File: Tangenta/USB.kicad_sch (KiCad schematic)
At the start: 31 parts, among them J12 907-211A1019D10200, J13 906-861A2116D10210, U8 USB2514B-I_M2, X1 X322524MOB4SI

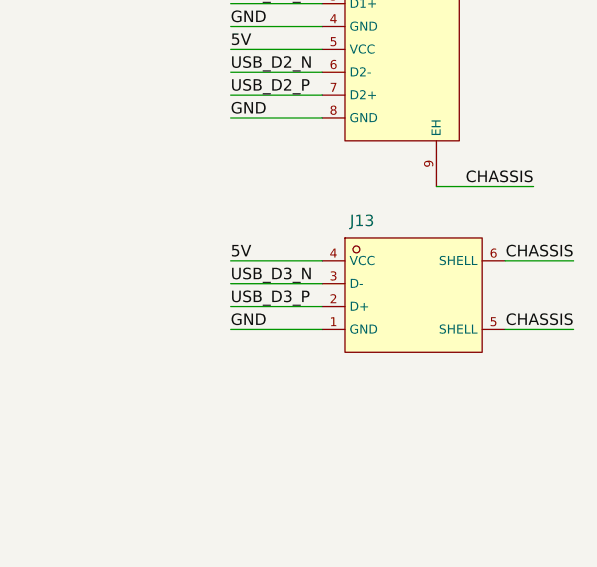
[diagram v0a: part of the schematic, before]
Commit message: ...
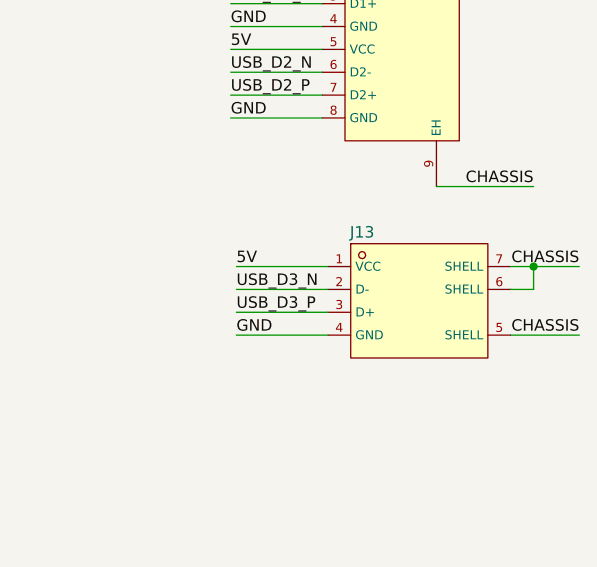
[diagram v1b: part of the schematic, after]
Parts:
- removed J13: 906-861A2116D10210, USB_VERTICAL:USB_Vertical, symbol USB_VERTICAL:906-861A2116D10210
- added J13: 906-151A1058D10200, USB_VERTICAL_BLUE:USB_VERTICAL_BLUE, symbol USB_VERTICAL_BLUE:906-151A1058D10200
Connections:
- net 5V: now also J13.1 (VCC)
- net CHASSIS: now also J13.5 (SHELL), J13.6 (SHELL), J13.7 (SHELL)
- net GNDREF: now also J13.4 (GND)
- net USB_D3_N: now also J13.2 (D-)
- net USB_D3_P: now also J13.3 (D+)
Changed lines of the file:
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@@
   (junction (at 114.3 177.8) (diameter 0) (color 0 0 0 0)
   )
+  (junction (at 279.4 88.9) (diameter 0) (color 0 0 0 0)
+  )
   (junction (at 95.25 168.91) (diameter 0) (color 0 0 0 0)
   )
@@
     (stroke (width 0) (type default))
   )
-  (wire (pts (xy 276.225 95.885) (xy 283.845 95.885))
+  (wire (pts (xy 276.86 96.52) (xy 284.48 96.52))
     (stroke (width 0) (type default))
   )
@@
     (stroke (width 0) (type default))
   )
-  (wire (pts (xy 276.225 88.265) (xy 283.845 88.265))
+  (wire (pts (xy 276.86 88.9) (xy 279.4 88.9))
     (stroke (width 0) (type default))
   )
@@
     (stroke (width 0) (type default))
   )
+  (wire (pts (xy 276.86 91.44) (xy 279.4 91.44))
+    (stroke (width 0) (type default))
+  )
   (wire (pts (xy 49.53 85.09) (xy 58.42 85.09))
     (stroke (width 0) (type default))
@@
     (stroke (width 0) (type default))
   )
-  (wire (pts (xy 245.745 95.885) (xy 255.905 95.885))
+  (wire (pts (xy 246.38 96.52) (xy 256.54 96.52))
     (stroke (width 0) (type default))
   )
@@
     (stroke (width 0) (type default))
   )
-  (wire (pts (xy 245.745 88.265) (xy 255.905 88.265))
+  (wire (pts (xy 246.38 88.9) (xy 256.54 88.9))
     (stroke (width 0) (type default))
   )
@@
     (stroke (width 0) (type default))
   )
-  (wire (pts (xy 245.745 90.805) (xy 255.905 90.805))
+  (wire (pts (xy 246.38 91.44) (xy 256.54 91.44))
     (stroke (width 0) (type default))
   )
@@
     (stroke (width 0) (type default))
   )
+  (wire (pts (xy 279.4 88.9) (xy 284.48 88.9))
+    (stroke (width 0) (type default))
+  )
   (wire (pts (xy 48.895 59.69) (xy 58.42 59.69))
     (stroke (width 0) (type default))
@@
     (stroke (width 0) (type default))
   )
-  (wire (pts (xy 245.745 93.345) (xy 255.905 93.345))
+  (wire (pts (xy 246.38 93.98) (xy 256.54 93.98))
     (stroke (width 0) (type default))
   )
@@
     (stroke (width 0) (type default))
   )
+  (wire (pts (xy 279.4 91.44) (xy 279.4 88.9))
+    (stroke (width 0) (type default))
+  )
   (wire (pts (xy 245.745 64.77) (xy 255.905 64.77))
     (stroke (width 0) (type default))
@@
     (effects (font (size 1.27 1.27)) (justify left bottom))
   )
-  (label "CHASSIS" (at 283.845 95.885 180) (fields_autoplaced)
-    (effects (font (size 1.27 1.27)) (justify right bottom))
-  )
-  (label "GND" (at 245.745 95.885 0) (fields_autoplaced)
+  (label "CHASSIS" (at 284.48 96.52 180) (fields_autoplaced)
+    (effects (font (size 1.27 1.27)) (justify right bottom))
+  )
+  (label "GND" (at 246.38 96.52 0) (fields_autoplaced)
     (effects (font (size 1.27 1.27)) (justify left bottom))
   )
@@
     (effects (font (size 1.27 1.27)) (justify right bottom))
   )
-  (label "USB_D3_N" (at 245.745 90.805 0) (fields_autoplaced)
+  (label "USB_D3_N" (at 246.38 91.44 0) (fields_autoplaced)
     (effects (font (size 1.27 1.27)) (justify left bottom))
   )
@@
     (effects (font (size 1.27 1.27)) (justify right bottom))
   )
-  (label "USB_D3_P" (at 245.745 93.345 0) (fields_autoplaced)
+  (label "USB_D3_P" (at 246.38 93.98 0) (fields_autoplaced)
     (effects (font (size 1.27 1.27)) (justify left bottom))
   )
@@
     (effects (font (size 1.27 1.27)) (justify left bottom))
   )
-  (label "5V" (at 245.745 88.265 0) (fields_autoplaced)
+  (label "5V" (at 246.38 88.9 0) (fields_autoplaced)
     (effects (font (size 1.27 1.27)) (justify left bottom))
   )
@@
     (effects (font (size 1.27 1.27)) (justify left bottom))
   )
-  (label "CHASSIS" (at 283.845 88.265 180) (fields_autoplaced)
+  (label "CHASSIS" (at 284.48 88.9 180) (fields_autoplaced)
     (effects (font (size 1.27 1.27)) (justify right bottom))
   )
@@
     )
   )
-  (symbol (lib_id "USB_VERTICAL:906-861A2116D10210") (at 266.065 90.805 0) (unit 1)
-    (in_bom yes) (on_board yes) (dnp no)
-    (property "Reference" "J13" (at 260.35 83.82 0)
-      (effects (font (size 1.27 1.27)))
-    )
-    (property "Value" "906-861A2116D10210" (at 266.065 83.82 0)
-      (effects (font (size 1.27 1.27)) hide)
-    )
-    (property "Footprint" "USB_VERTICAL:USB_Vertical" (at 269.875 106.045 0)
-      (effects (font (size 1.27 1.27) italic) hide)
-    )
-    (property "Datasheet" "https://atta.szlcsc.com/upload/public/pdf/source/20210526/C2763350_E0D561271332FF88E1B9AF264603FE9E.pdf" (at 257.175 108.585 0)
-      (effects (font (size 1.27 1.27)) (justify left) hide)
-    )
-    (property "LCSC" "C2763350" (at 262.255 103.505 0)
-      (effects (font (size 1.27 1.27)) hide)
-    )
-    (pin "1")
-    (pin "2")
-    (pin "3")
-    (pin "4")
-    (pin "5")
-    (pin "6")
-    (instances
-      (project "Tangenta"
-        (path "/358d1bcf-7599-4352-8c4d-baa18a5f09e6/b1871a4d-6a35-44e2-a9a2-9a4af684371d"
-          (reference "J13") (unit 1)
-        )
-      )
-    )
-  )
   (symbol (lib_id "Device:C_Small") (at 206.375 93.98 180) (unit 1)
     (in_bom yes) (on_board yes) (dnp no)
@@
         )
       )
+    )
+  )
+  (symbol (lib_id "USB_VERTICAL_BLUE:906-151A1058D10200") (at 266.7 93.98 0) (unit 1)
+    (in_bom yes) (on_board yes) (dnp no)
+    (property "Reference" "J13" (at 260.35 85.09 0)
+      (effects (font (size 1.27 1.27)))
+    )
+    (property "Value" "906-151A1058D10200" (at 266.7 100.33 0)
+      (effects (font (size 1.27 1.27)) hide)
+    )
+    (property "Footprint" "USB_VERTICAL_BLUE:USB_VERTICAL_BLUE" (at 267.589 108.585 0)
+      (effects (font (size 1.27 1.27) italic) hide)
+    )
+    (property "Datasheet" "https://item.szlcsc.com/2892439.html" (at 248.539 106.299 0)
+      (effects (font (size 1.27 1.27)) (justify left) hide)
+    )
+    (property "LCSC" "C2763227" (at 253.492 104.267 0)
+      (effects (font (size 1.27 1.27)) hide)
+    )
+    (pin "1")
+    (pin "2")
+    (pin "3")
+    (pin "4")
+    (pin "5")
+    (pin "6")
+    (pin "7")
+    (instances
+      (project "Tangenta"
+        (path "/358d1bcf-7599-4352-8c4d-baa18a5f09e6/b1871a4d-6a35-44e2-a9a2-9a4af684371d"
+          (reference "J13") (unit 1)
+        )
+      )
